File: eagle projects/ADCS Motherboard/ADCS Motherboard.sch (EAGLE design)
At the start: 142 parts, among them J1 HDR_10_EZFET_DEBUGGER, J11 CNC_3221-10-0300-00, J3 CNC_3221-10-0300-00, J5 CNC_3221-10-0300-00, J7 TE-1734829-3, Q1 PMV16XN, Q2 IRLML6246TRPBF, Q3 IRLML2246TRPBF, U1 MSP430F5529IPN, U10 TSV991AILT, U2 TSV991AILT, U3 ADS7841E_2K5, U4 TSV991AILT, U7 HMC1053, U9 BMX160, Y1 32.768kHz, Y2 CSTCR4M00G15L99, Y3 32.768kHz

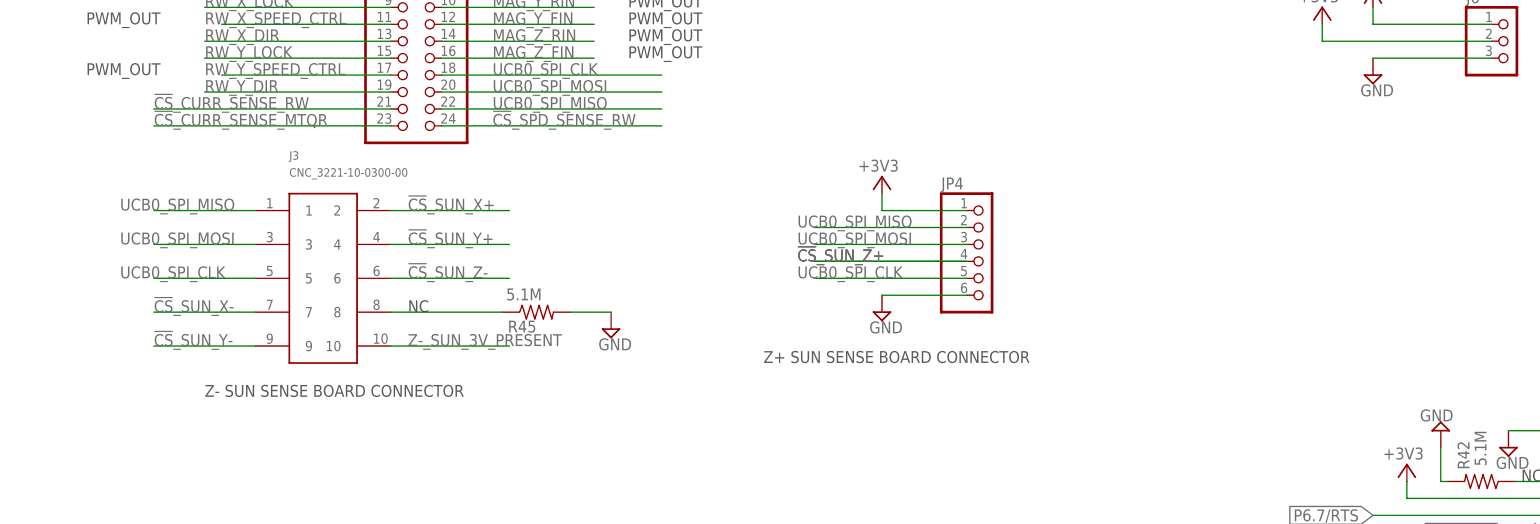
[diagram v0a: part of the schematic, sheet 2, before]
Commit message: Rev B almost ready
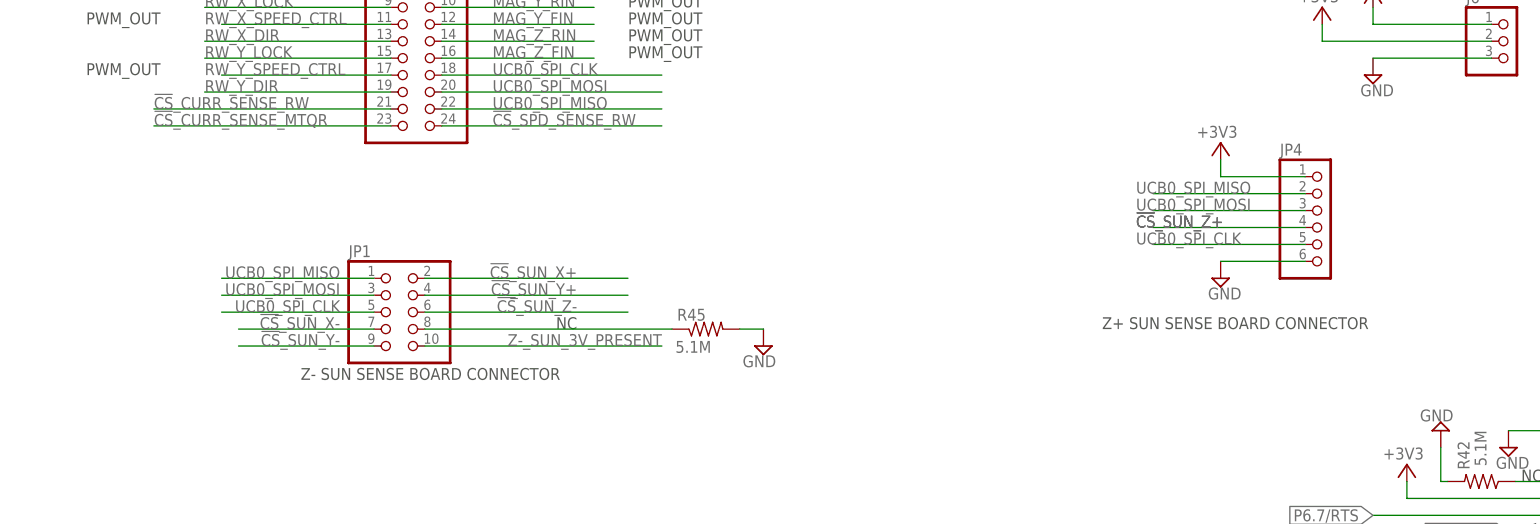
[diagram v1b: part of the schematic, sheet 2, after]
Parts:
- removed J3: CNC_3221-10-0300-00, my_library:CNC_3221-10-0300-00
- added JP1: (no value), pinhead:PINHD-2X5
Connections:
- net !CS!_SUN_X+: now also JP1.2; no longer J3.2
- net !CS!_SUN_X-: now also JP1.7; no longer J3.7
- net !CS!_SUN_Y+: now also JP1.4; no longer J3.4
- net !CS!_SUN_Y-: now also JP1.9; no longer J3.9
- net !CS!_SUN_Z-: now also JP1.6; no longer J3.6
- net N$58: now also JP1.8; no longer J3.8
- net UCB0_SPI_CLK: now also JP1.5; no longer J3.5
- net UCB0_SPI_MISO: now also JP1.1; no longer J3.1
- net UCB0_SPI_MOSI: now also JP1.3; no longer J3.3
- net Z-_SUN_3V_PRESENT: now also JP1.10; no longer J3.10
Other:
- moved on the sheet: JP4, R45
